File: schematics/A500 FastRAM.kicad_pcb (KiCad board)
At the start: 2 copper layers, 87.6 x 87.6 mm, 31 parts, among them J1 Microsemi_FlashPro-JTAG-10, U1 68000 Boardside, U10 TPS7333QP, U2 68000 Socket, U3 ATF1502ASV-15JU44, U4 74157, U5 74157, U6 IS41LV16100D, U7 IS41LV16100D, U8 IS41LV16100D, U9 IS41LV16100D

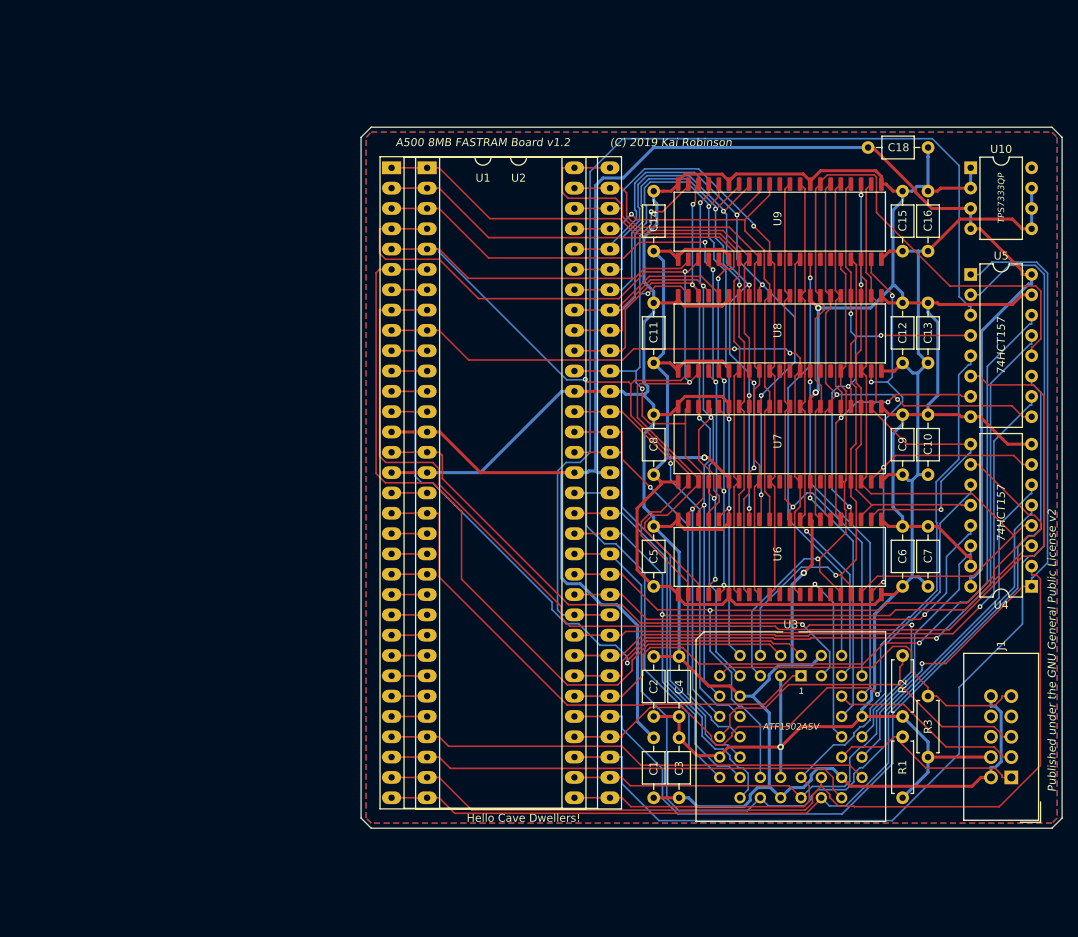
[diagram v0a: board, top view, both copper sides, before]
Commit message: Add files via upload
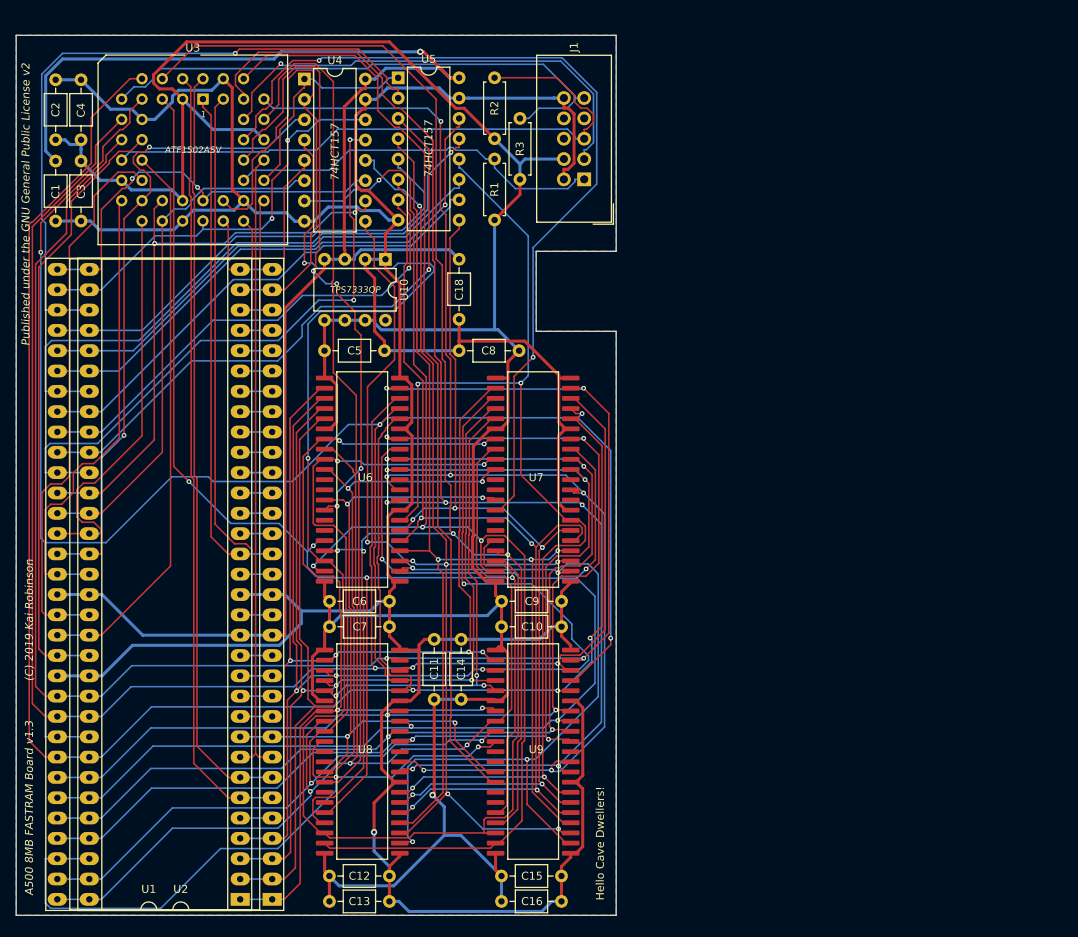
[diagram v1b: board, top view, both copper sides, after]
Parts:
- moved U4 110.8 mm to (111.0, 24.5), turned to 0 degrees
- moved C1 103.9 mm to (79.9, 34.7)
- moved C2 103.9 mm to (79.9, 24.6)
- moved C4 103.9 mm to (83.1, 24.6)
- moved U3 103.9 mm to (98.3, 27.0)
- moved C3 103.9 mm to (83.1, 34.7)
- moved C13 100.6 mm to (114.2, 127.3), turned to 0 degrees
- moved C16 97.2 mm to (135.7, 127.3), turned to 0 degrees
- moved C12 96.2 mm to (114.2, 124.1), turned to 0 degrees
- moved U2 93.5 mm to (107.0, 127.0), turned to 180 degrees
- moved U1 93.4 mm to (103.0, 127.0), turned to 180 degrees
- moved C15 92.8 mm to (135.7, 124.1), turned to 0 degrees
- moved J1 91.9 mm to (146.0, 37.0)
- moved R1 88.4 mm to (134.8, 42.1)
- moved R2 88.4 mm to (134.8, 31.9)
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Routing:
- net /CPU_D13: track 103.1 -> 241.5 mm, vias 3 -> 4
- net /DRAM_A1: track 63.1 -> 196.7 mm, vias 1 -> 4
- net /CPU_D14: track 92.7 -> 225.3 mm, vias 4 -> 3
- net /CPU_D12: track 114.0 -> 240.6 mm
- net /CPU_D15: track 96.7 -> 211.6 mm
- net /DRAM_A2: track 76.0 -> 184.5 mm, vias 0 -> 2
- net /DRAM_A0: track 65.5 -> 169.5 mm, vias 1 -> 4
- net /DRAM_UCAS: track 66.0 -> 166.8 mm, vias 1 -> 5
- net /DRAM_LCAS: track 72.4 -> 159.9 mm, vias 1 -> 6
- net /DRAM_A3: track 71.2 -> 156.8 mm
- net /DRAM_A6: track 62.7 -> 147.4 mm, vias 4 -> 3
- net /DRAM_A4: track 62.6 -> 145.0 mm, vias 1 -> 5
- net /DRAM_RAS1: track 32.2 -> 110.4 mm, vias 1 -> 2
- net /CPU_A4: track 106.2 -> 28.1 mm
- net /CPU_D5: track 80.3 -> 156.0 mm, vias 2 -> 3
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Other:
- board size 87.6 x 87.6 mm -> 75 x 110 mm
- board text added: "A500 8MB FASTRAM Board v1.3"
- board text removed: "A500 8MB FASTRAM Board v1.2"
